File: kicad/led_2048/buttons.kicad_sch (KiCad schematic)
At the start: 32 parts, among them SW10 Up, SW3 Right, SW4 Left, SW5 Down, SW6 B button, SW7 A button, SW8 R button, SW9 L button

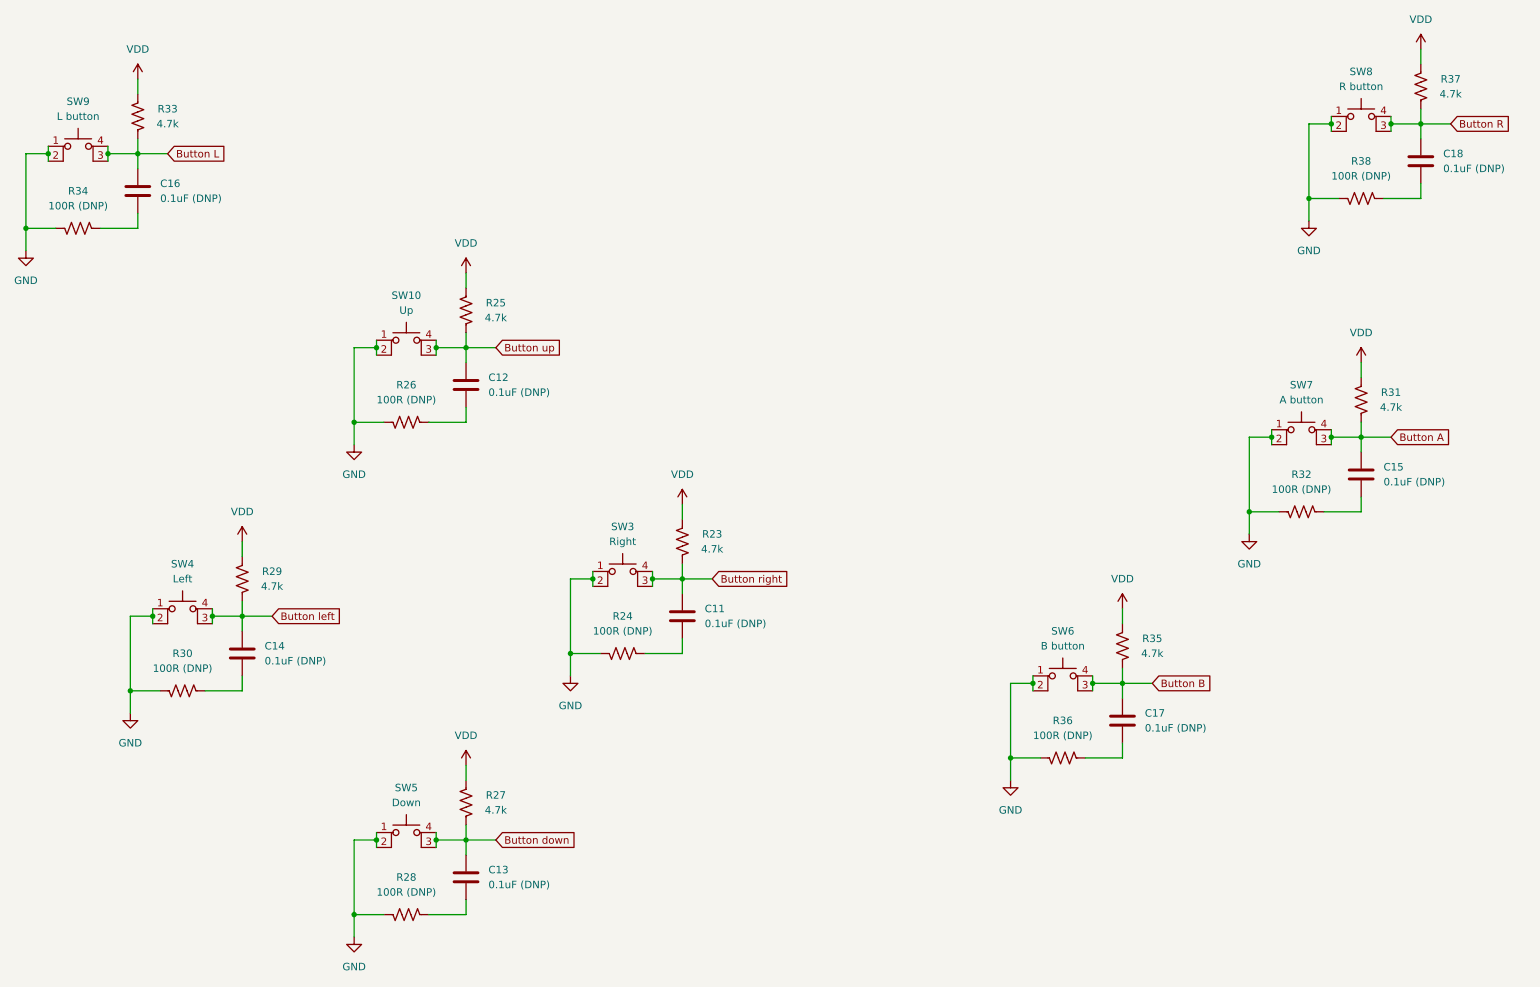
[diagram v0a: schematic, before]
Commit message: finished layout
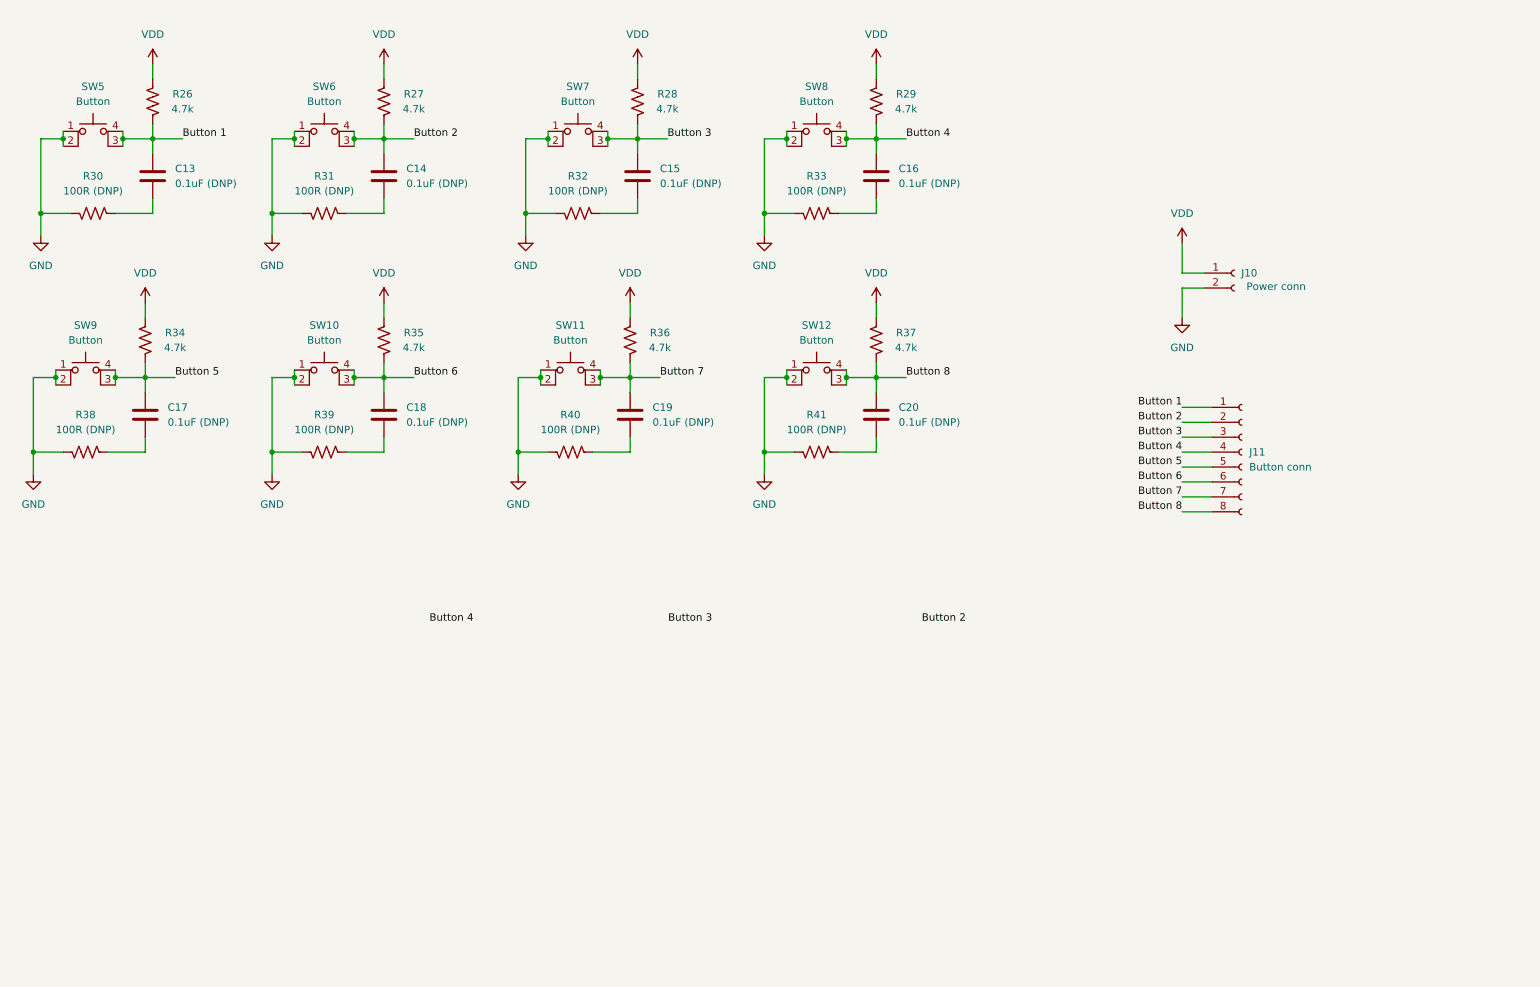
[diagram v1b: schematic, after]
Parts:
- removed SW3: Right, 2048_footprints:SW_TL1105SPF160Q, symbol Switch:SW_MEC_5E
- removed SW4: Left, 2048_footprints:SW_TL1105SPF160Q, symbol Switch:SW_MEC_5E
- added J10: Power conn, Connector_PinSocket_2.00mm:PinSocket_1x02_P2.00mm_Vertical, symbol Connector:Conn_01x02_Socket
- added J11: Button conn, Connector_PinSocket_2.00mm:PinSocket_1x08_P2.00mm_Vertical, symbol Connector:Conn_01x08_Socket
- added SW11, SW12: Button, 2048_footprints:SW_TL1105SPF160Q, symbol Switch:SW_MEC_5E
- SW10: value Up -> Button
- SW5: value Down -> Button
- SW6: value B button -> Button
- SW7: value A button -> Button
- SW8: value R button -> Button
- SW9: value L button -> Button
- renumbered C14 to C13, C13 to C14, C16 to C15, C18 to C16, C12 to C17, C11 to C18, C17 to C19, C15 to C20, R29 to R26, R33 to R28, R37 to R29, R28 to R31, R34 to R32, R38 to R33, R25 to R34, R23 to R35, R35 to R36, R31 to R37, R26 to R38, R24 to R39, R36 to R40, R32 to R41
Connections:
- net Button left is gone; now on net Button 1: C13.1, R26.1
- net GND: now also J10.2 (Pin_2), SW11.1, SW11.2, SW12.1, SW12.2
- net VDD: now also J10.1 (Pin_1)
- net Button A renamed Button 3
- net Button 3: now also C15.1, R28.1, J11.3 (Pin_3); no longer C20.1, R37.1
- net Button B renamed Button 2
- net Button 2: now also C14.1, R27.1, J11.2 (Pin_2); no longer C19.1, R36.1
- net Button L renamed Button 5
- net Button 5: now also C17.1, R34.1, J11.5 (Pin_5); no longer C15.1, R28.1
- net Button R renamed Button 4
- net Button 4: now also J11.4 (Pin_4)
- net Button down renamed Button 1
- net Button 1: now also J11.1 (Pin_1); no longer C14.1, R27.1
- net Button right renamed Button 6
- net Button 6: now also SW10.3 (K), SW10.4 (A), J11.6 (Pin_6)
- removed net Button up: C17.1, R34.1, SW10.3 (K), SW10.4 (A)
- new net Button 7: C19.1, J11.7 (Pin_7), R36.1, SW11.3 (K), SW11.4 (A)
- new net Button 8: C20.1, J11.8 (Pin_8), R37.1, SW12.3 (K), SW12.4 (A)
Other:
- moved on the sheet: C13, C14, C15, C16, C17, C18, C19, C20, R26, R27, R28, R29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
